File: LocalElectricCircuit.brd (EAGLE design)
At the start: 160 x 100 mm, 45 parts, among them IC1 PIC32MX360F512L, J1 Prog. Port, J3 Prog. Port, T1 PN100, U1 ADS1118, U2 ADS1118

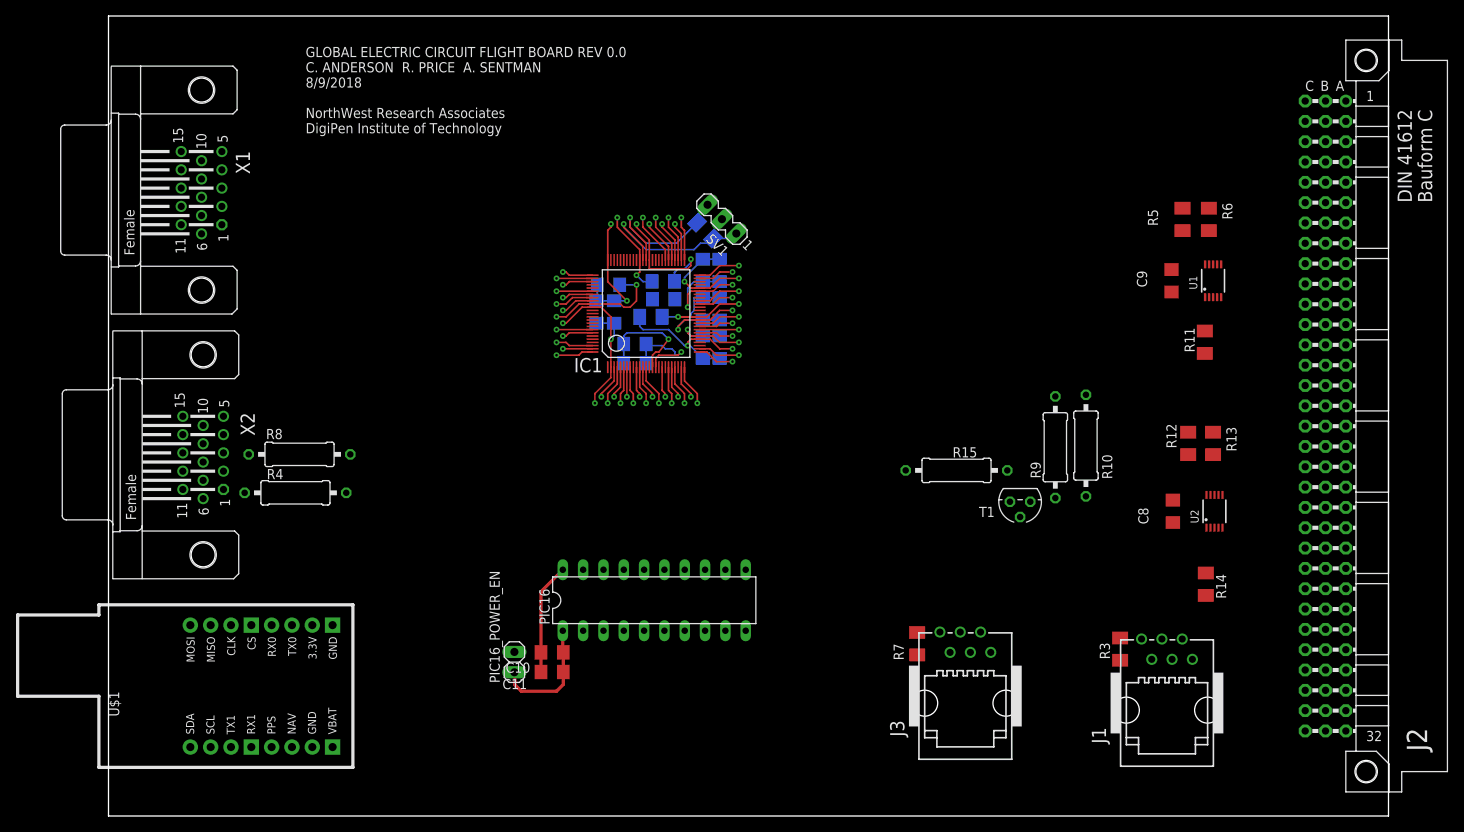
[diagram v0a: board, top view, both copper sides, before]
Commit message: Auto router did a goody
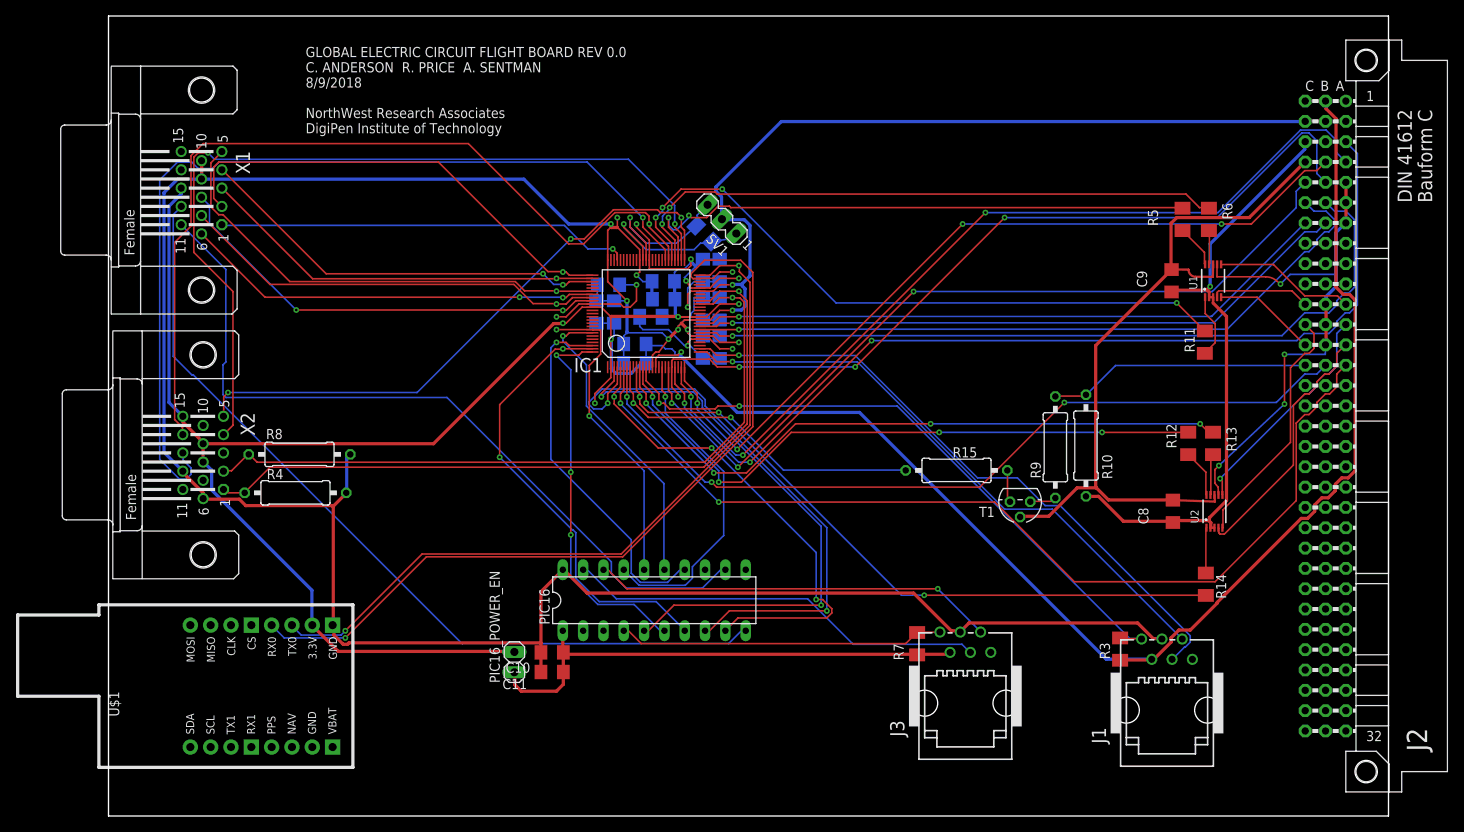
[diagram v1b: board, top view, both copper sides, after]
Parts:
- moved R1 0.41 mm to (74.5, 22.8)
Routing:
- net GND_3V3: track 95.5 -> 454.6 mm
- net +3V3: track 87.2 -> 416.7 mm
- net CHARGE_PROBE_0: track 4.67 -> 122.7 mm, vias 1 -> 2
- net TEMP_3: track 5.00 -> 122.0 mm, vias 1 -> 3
- net I2C_SCL: track 6.46 -> 114.6 mm
- net PIC16_TX: track 0.00 -> 106.2 mm
- net TEMP_2: track 4.20 -> 109.4 mm, vias 1 -> 3
- net U1RX: track 4.83 -> 107.4 mm, vias 1 -> 2
- net I2C_SDA: track 5.49 -> 107.5 mm
- net U2RX: track 4.43 -> 106.1 mm, vias 1 -> 2
- net I_1_L: track 4.03 -> 104.1 mm, vias 1 -> 4
- net CHARGE_PROBE_1: track 3.70 -> 102.5 mm, vias 1 -> 3
- net I_1_H: track 4.67 -> 103.2 mm, vias 1 -> 3
- net PIC16_RX: track 0.00 -> 98.3 mm
- net TEMP_1: track 5.16 -> 101.4 mm, vias 1 -> 4
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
